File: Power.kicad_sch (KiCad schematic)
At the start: 6 parts, among them U2 AZ1117-3.3, U7 AZ1117-5.0

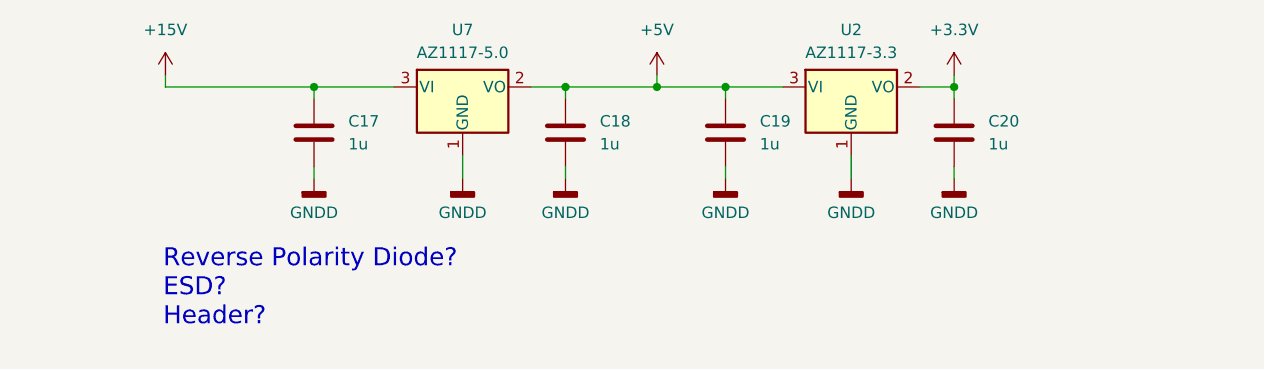
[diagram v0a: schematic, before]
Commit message: 90% schematic first layout
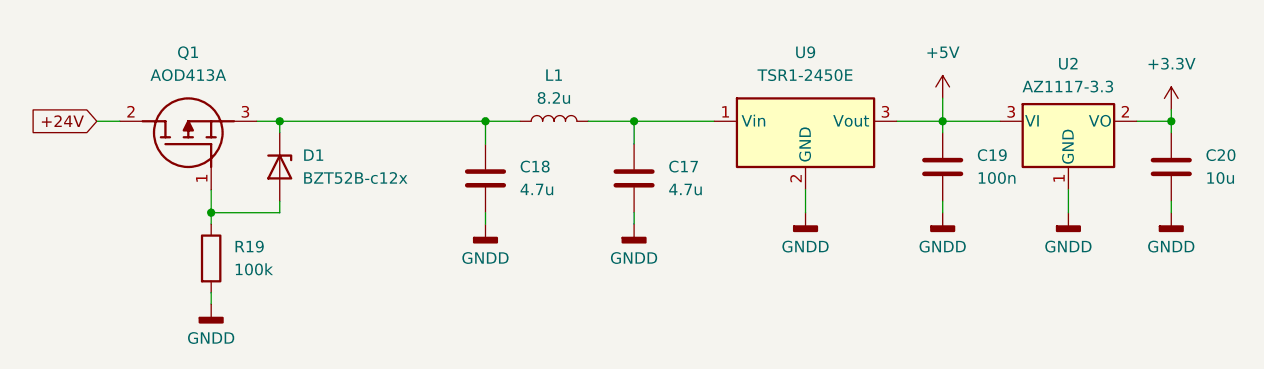
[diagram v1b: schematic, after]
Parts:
- removed U7: AZ1117-5.0, Package_TO_SOT_SMD:SOT-223-3_TabPin2, symbol Regulator_Linear:AZ1117-5.0
- added D1: BZT52B-c12x, Diode_SMD:D_SOD-123F, symbol Diode:BZT52Bxx
- added L1: 8.2u, Inductor_SMD:L_6.3x6.3_H3, symbol Device:L
- added Q1: AOD413A, AOD413A, symbol AOD413A:AOD413A
- added R19: 100k, Resistor_SMD:R_0805_2012Metric_Pad1.20x1.40mm_HandSolder, symbol Device:R
- added U9: TSR1-2450E, Converter_DCDC:Converter_DCDC_TRACO_TSR1-xxxxE_THT, symbol Regulator_Switching:TSR1-2450E
- C17, C18: value 1u -> 4.7u
- C19: value 1u -> 100n
- C20: value 1u -> 10u
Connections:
- net +5V: now also U9.3 (Vout); no longer C18.2
- net GNDD: now also R19.2, U9.2 (GND)
- net +15V: no longer names the net of C17.2
- net +15V: now also L1.2, U9.1 (Vin)
- new net: D1.2 (A), Q1.1 (G), R19.1
- new net: C18.2, D1.1 (K), L1.1, Q1.3 (S)
- new net +24V: Q1.2 (D)
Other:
- note removed: "Reverse Polarity Diode? ESD? Header?"
- moved on the sheet: C19, C20, U2
